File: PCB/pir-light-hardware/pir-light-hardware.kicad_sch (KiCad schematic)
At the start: 44 parts, among them J1 ZH1.5-3, J2 ZH1.5-3, Q1 AON7240, Q2 NPN, Q3 PNP, Q4 PNP, U1 M74VHC1GT08DFT2G, U2 LMV331IDCKR, U3 AS312

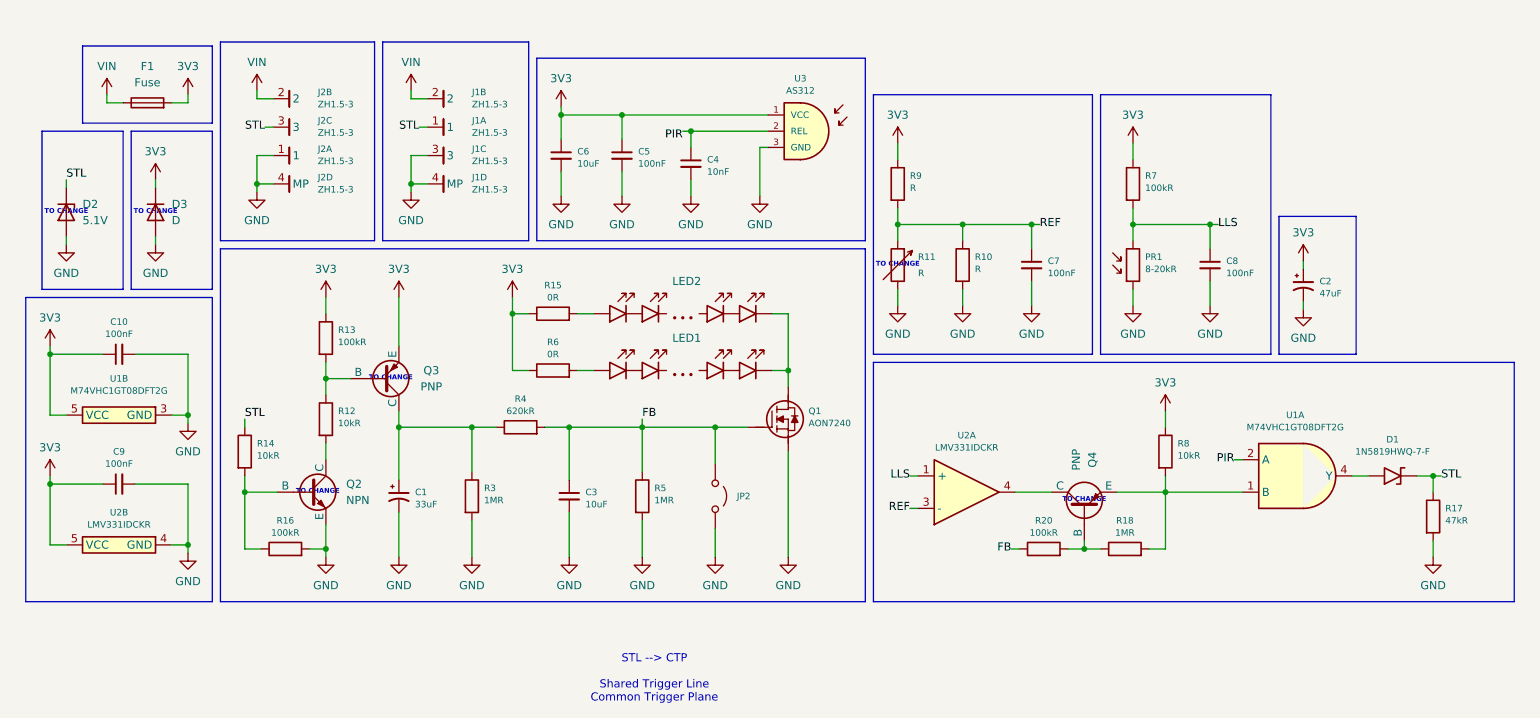
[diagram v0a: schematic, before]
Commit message: docs: update readme
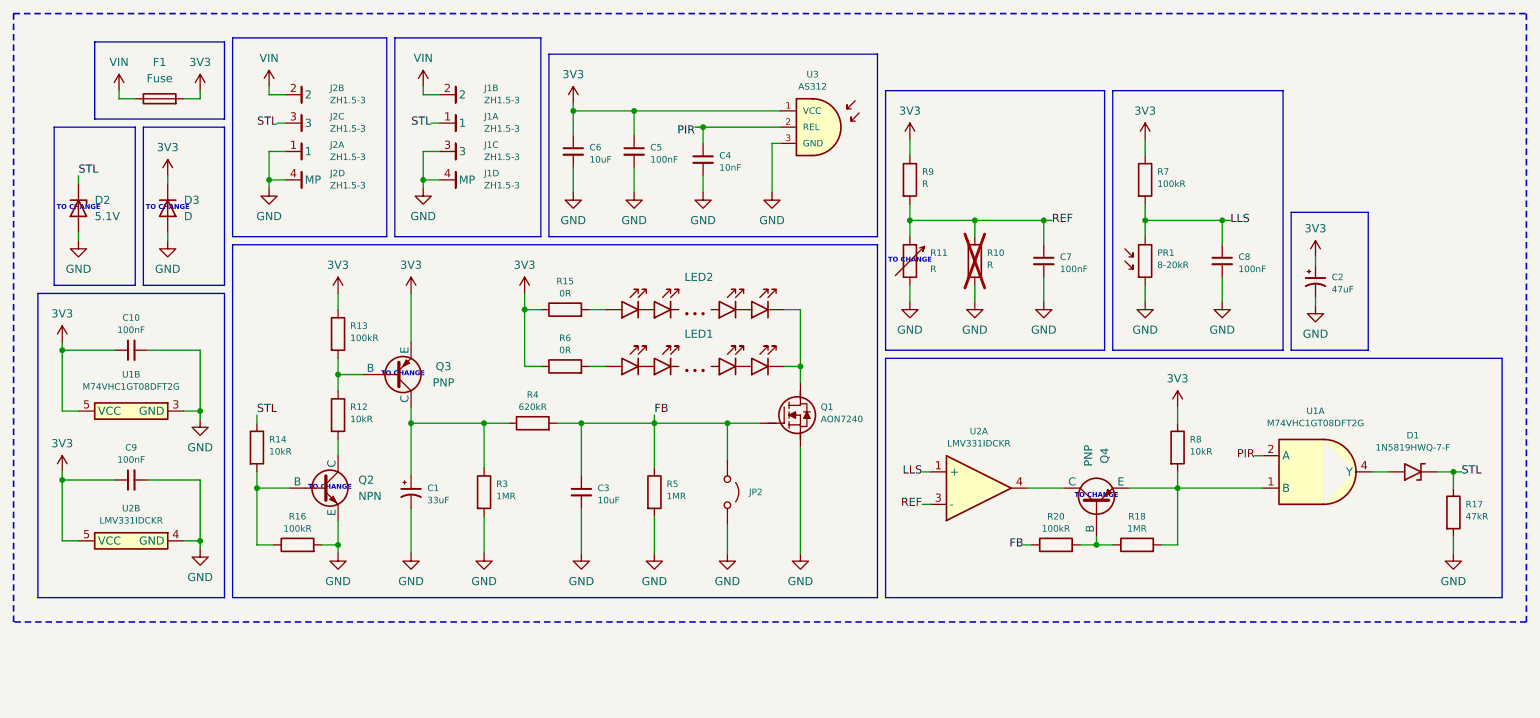
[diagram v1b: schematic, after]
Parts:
- R10: now not fitted
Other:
- note removed: "STL --> CTP Shared Trigger Line Common Trigger Plane"
- company: (none) -> Designed by Marcin Trzmiel
- title: (none) -> PIR motion-controlled light module
- moved on the sheet: C1, C10, C2, C3, C4, C5, C6, C7, C8, C9, D1, D2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
